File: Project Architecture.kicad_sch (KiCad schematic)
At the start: 0 parts

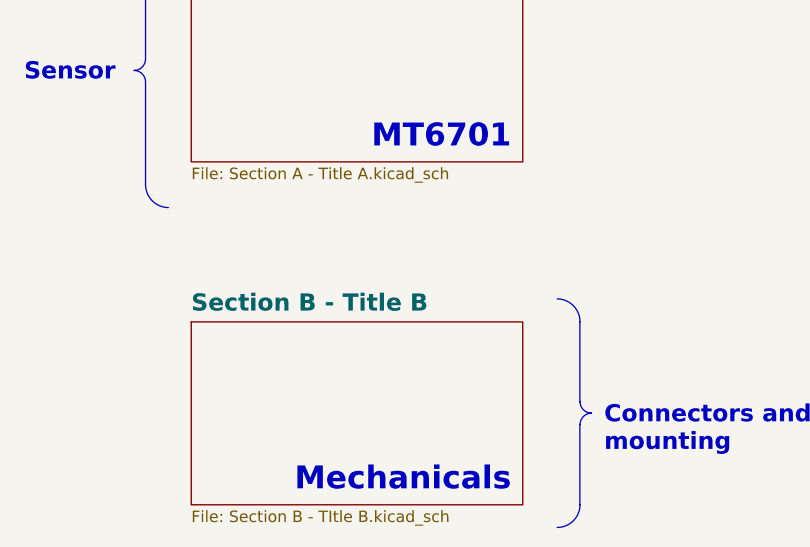
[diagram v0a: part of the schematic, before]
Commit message: [PCB] added basic layout
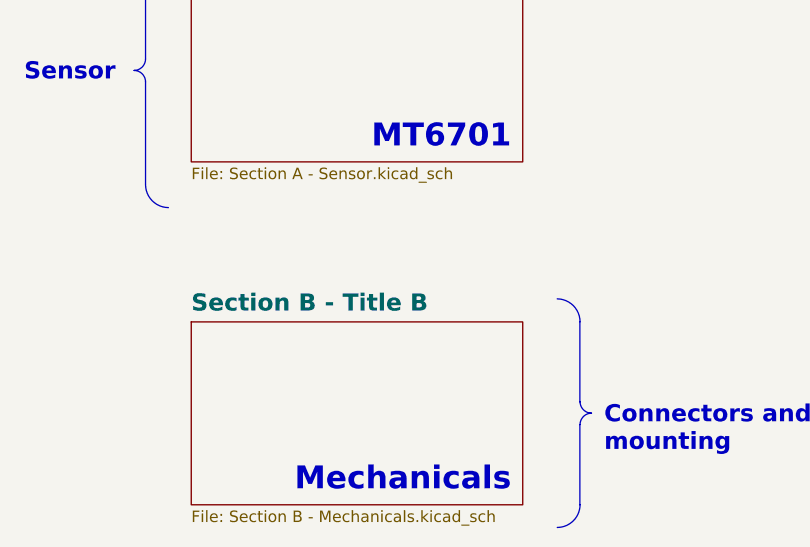
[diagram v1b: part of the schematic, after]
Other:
- sheet Section A - Title A: file Section A - Title A.kicad_sch -> Section A - Sensor.kicad_sch
- sheet Section B - Title B: file Section B - TItle B.kicad_sch -> Section B - Mechanicals.kicad_sch
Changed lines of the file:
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@@
 			)
 		)
-		(property "Sheetfile" "Section B - TItle B.kicad_sch"
+		(property "Sheetfile" "Section B - Mechanicals.kicad_sch"
 			(at 190.5 135.2046 0)
 			(effects
@@
 			)
 		)
-		(property "Sheetfile" "Section A - Title A.kicad_sch"
+		(property "Sheetfile" "Section A - Sensor.kicad_sch"
 			(at 190.5 97.1046 0)
 			(effects
